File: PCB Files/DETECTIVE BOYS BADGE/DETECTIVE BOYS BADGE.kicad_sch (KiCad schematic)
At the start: 39 parts, among them J1 Jack 3.5mm, J2 ICSP, SW1 SPDT_PCM12, SW2 Pushbutton, U1 NRF24L01_Breakout, U2 MIC5205-3.3YM5, U3 TP4056, U4 LM358, U5 ATmega328P-A, X1 Resonator 8MHz

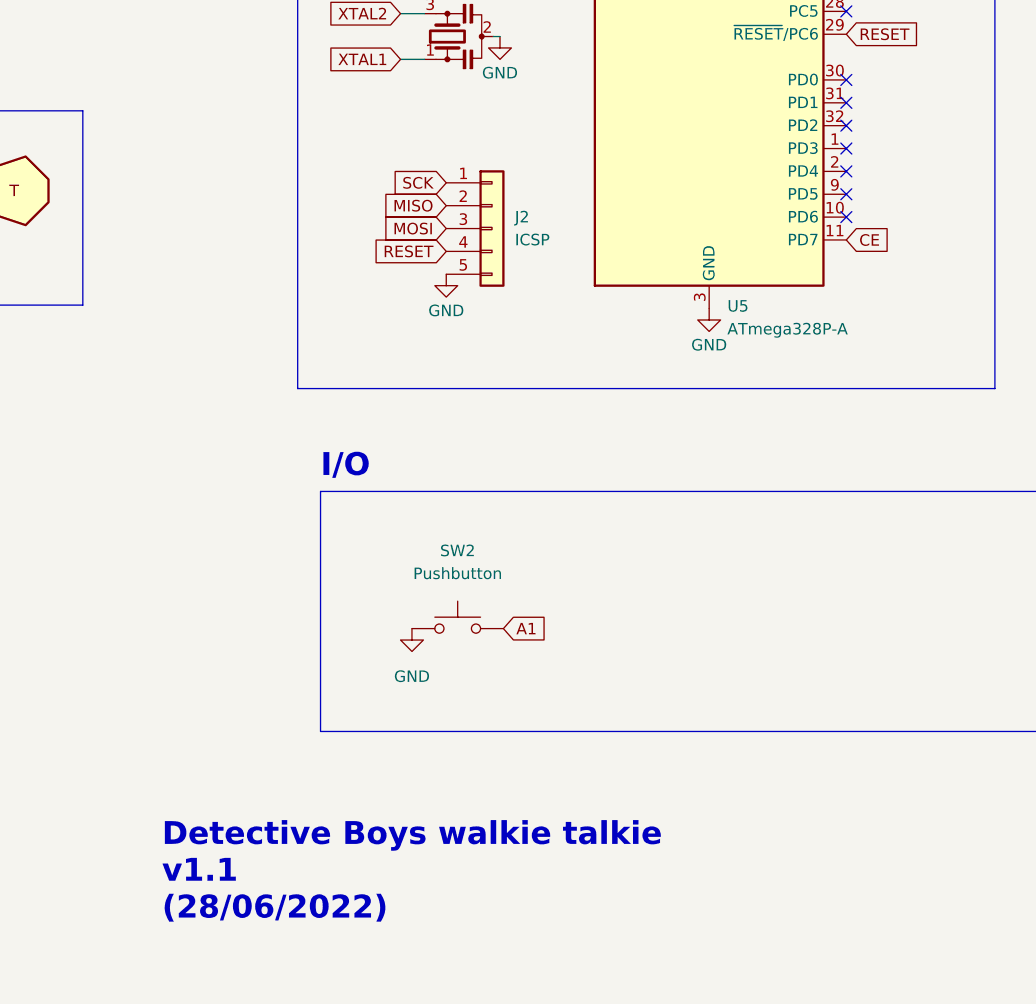
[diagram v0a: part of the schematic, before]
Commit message: Updated Schematic PDF file
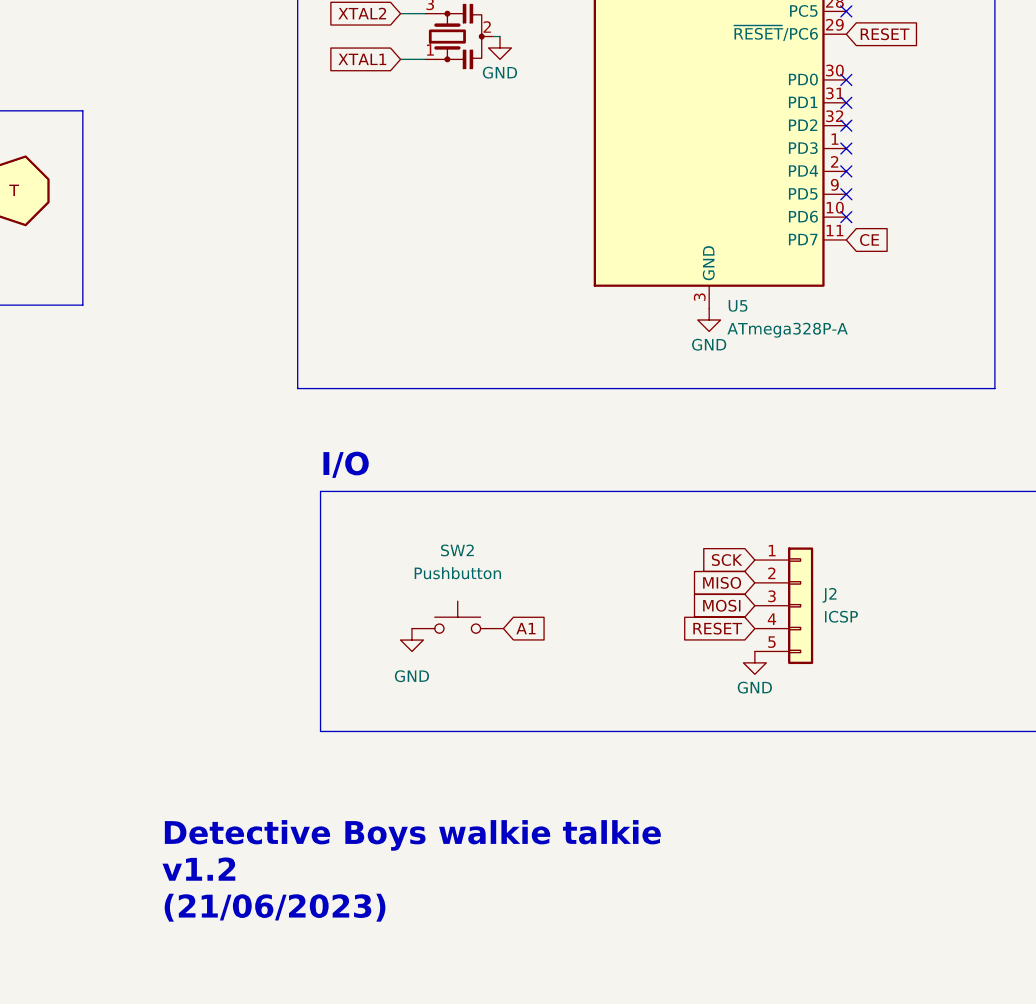
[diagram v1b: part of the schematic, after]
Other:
- note added: "Detective Boys walkie talkie v1.2 (21/06/2023)"
- note removed: "Detective Boys walkie talkie v1.1 (28/06/2022)"
- moved on the sheet: J2
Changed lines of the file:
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@@
     (effects (font (size 2.54 2.54) (thickness 0.508) bold) (justify left bottom))
   )
-  (text "Detective Boys walkie talkie\nv1.1\n(28/06/2022)" (at 177.9643 179.9857 0)
+  (text "Detective Boys walkie talkie\nv1.2\n(21/06/2023)" (at 177.9643 179.9857 0)
     (effects (font (size 2.54 2.54) (thickness 0.508) bold) (justify left bottom))
   )
@@
     )
   )
-  (global_label "MISO" (shape input) (at 209.55 100.33 180) (fields_autoplaced)
-    (effects (font (size 1.27 1.27)) (justify right))
-    (property "Intersheet References" "${INTERSHEET_REFS}" (id 0) (at 202.5407 100.2506 0)
+  (global_label "MISO" (shape input) (at 243.84 142.24 180) (fields_autoplaced)
+    (effects (font (size 1.27 1.27)) (justify right))
+    (property "Intersheet References" "${INTERSHEET_REFS}" (id 0) (at 236.8307 142.1606 0)
       (effects (font (size 1.27 1.27)) (justify right) hide)
     )
@@
     )
   )
-  (global_label "SCK" (shape input) (at 209.55 97.79 180) (fields_autoplaced)
-    (effects (font (size 1.27 1.27)) (justify right))
-    (property "Intersheet References" "${INTERSHEET_REFS}" (id 0) (at 203.3874 97.7106 0)
+  (global_label "SCK" (shape input) (at 243.84 139.7 180) (fields_autoplaced)
+    (effects (font (size 1.27 1.27)) (justify right))
+    (property "Intersheet References" "${INTERSHEET_REFS}" (id 0) (at 237.6774 139.6206 0)
       (effects (font (size 1.27 1.27)) (justify right) hide)
     )
@@
     )
   )
-  (global_label "MOSI" (shape input) (at 209.55 102.87 180) (fields_autoplaced)
-    (effects (font (size 1.27 1.27)) (justify right))
-    (property "Intersheet References" "${INTERSHEET_REFS}" (id 0) (at 202.5407 102.7906 0)
+  (global_label "MOSI" (shape input) (at 243.84 144.78 180) (fields_autoplaced)
+    (effects (font (size 1.27 1.27)) (justify right))
+    (property "Intersheet References" "${INTERSHEET_REFS}" (id 0) (at 236.8307 144.7006 0)
       (effects (font (size 1.27 1.27)) (justify right) hide)
     )
@@
     )
   )
-  (global_label "RESET" (shape input) (at 209.55 105.41 180) (fields_autoplaced)
-    (effects (font (size 1.27 1.27)) (justify right))
-    (property "Intersheet References" "${INTERSHEET_REFS}" (id 0) (at 201.3917 105.4894 0)
+  (global_label "RESET" (shape input) (at 243.84 147.32 180) (fields_autoplaced)
+    (effects (font (size 1.27 1.27)) (justify right))
+    (property "Intersheet References" "${INTERSHEET_REFS}" (id 0) (at 235.6817 147.3994 0)
       (effects (font (size 1.27 1.27)) (justify right) hide)
     )
@@
     (pin "8")
   )
-  (symbol (lib_id "power:GND") (at 209.55 107.95 0) (unit 1)
-    (in_bom yes) (on_board yes)
-    (property "Reference" "#PWR030" (id 0) (at 209.55 114.3 0)
-      (effects (font (size 1.27 1.27)) hide)
-    )
-    (property "Value" "GND" (id 1) (at 209.55 112.014 0))
-    (property "Footprint" "" (id 2) (at 209.55 107.95 0)
-      (effects (font (size 1.27 1.27)) hide)
-    )
-    (property "Datasheet" "" (id 3) (at 209.55 107.95 0)
+  (symbol (lib_id "power:GND") (at 243.84 149.86 0) (unit 1)
+    (in_bom yes) (on_board yes)
+    (property "Reference" "#PWR030" (id 0) (at 243.84 156.21 0)
+      (effects (font (size 1.27 1.27)) hide)
+    )
+    (property "Value" "GND" (id 1) (at 243.84 153.924 0))
+    (property "Footprint" "" (id 2) (at 243.84 149.86 0)
+      (effects (font (size 1.27 1.27)) hide)
+    )
+    (property "Datasheet" "" (id 3) (at 243.84 149.86 0)
       (effects (font (size 1.27 1.27)) hide)
     )
@@
     (pin "1")
   )
-  (symbol (lib_id "Connector_Generic:Conn_01x05") (at 214.63 102.87 0) (unit 1)
-    (in_bom yes) (on_board yes) (fields_autoplaced)
-    (property "Reference" "J2" (id 0) (at 217.17 101.5999 0)
-      (effects (font (size 1.27 1.27)) (justify left))
-    )
-    (property "Value" "ICSP" (id 1) (at 217.17 104.1399 0)
-      (effects (font (size 1.27 1.27)) (justify left))
-    )
-    (property "Footprint" "Connector_FFC-FPC:Molex_200528-0050_1x05-1MP_P1.00mm_Horizontal" (id 2) (at 214.63 102.87 0)
-      (effects (font (size 1.27 1.27)) hide)
-    )
-    (property "Datasheet" "~" (id 3) (at 214.63 102.87 0)
-      (effects (font (size 1.27 1.27)) hide)
-    )
+  (symbol (lib_id "Connector_Generic:Conn_01x05") (at 248.92 144.78 0) (unit 1)
+    (in_bom yes) (on_board yes) (fields_autoplaced)
+    (property "Reference" "J2" (id 0) (at 251.46 143.5099 0)
+      (effects (font (size 1.27 1.27)) (justify left))
+    )
+    (property "Value" "ICSP" (id 1) (at 251.46 146.0499 0)
+      (effects (font (size 1.27 1.27)) (justify left))
+    )
+    (property "Footprint" "Connector_FFC-FPC:Molex_200528-0050_1x05-1MP_P1.00mm_Horizontal" (id 2) (at 248.92 144.78 0)
+      (effects (font (size 1.27 1.27)) hide)
+    )
+    (property "Datasheet" "~" (id 3) (at 248.92 144.78 0)
+      (effects (font (size 1.27 1.27)) hide)
+    )
